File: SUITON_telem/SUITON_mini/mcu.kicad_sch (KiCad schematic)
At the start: 24 parts, among them J2 USB_C_Receptacle_USB2.0_14P, J4 Conn_01x06_Pin, U5 STM32F405RGT6, X1 ABM3B-8.000MHZ-10-1UT

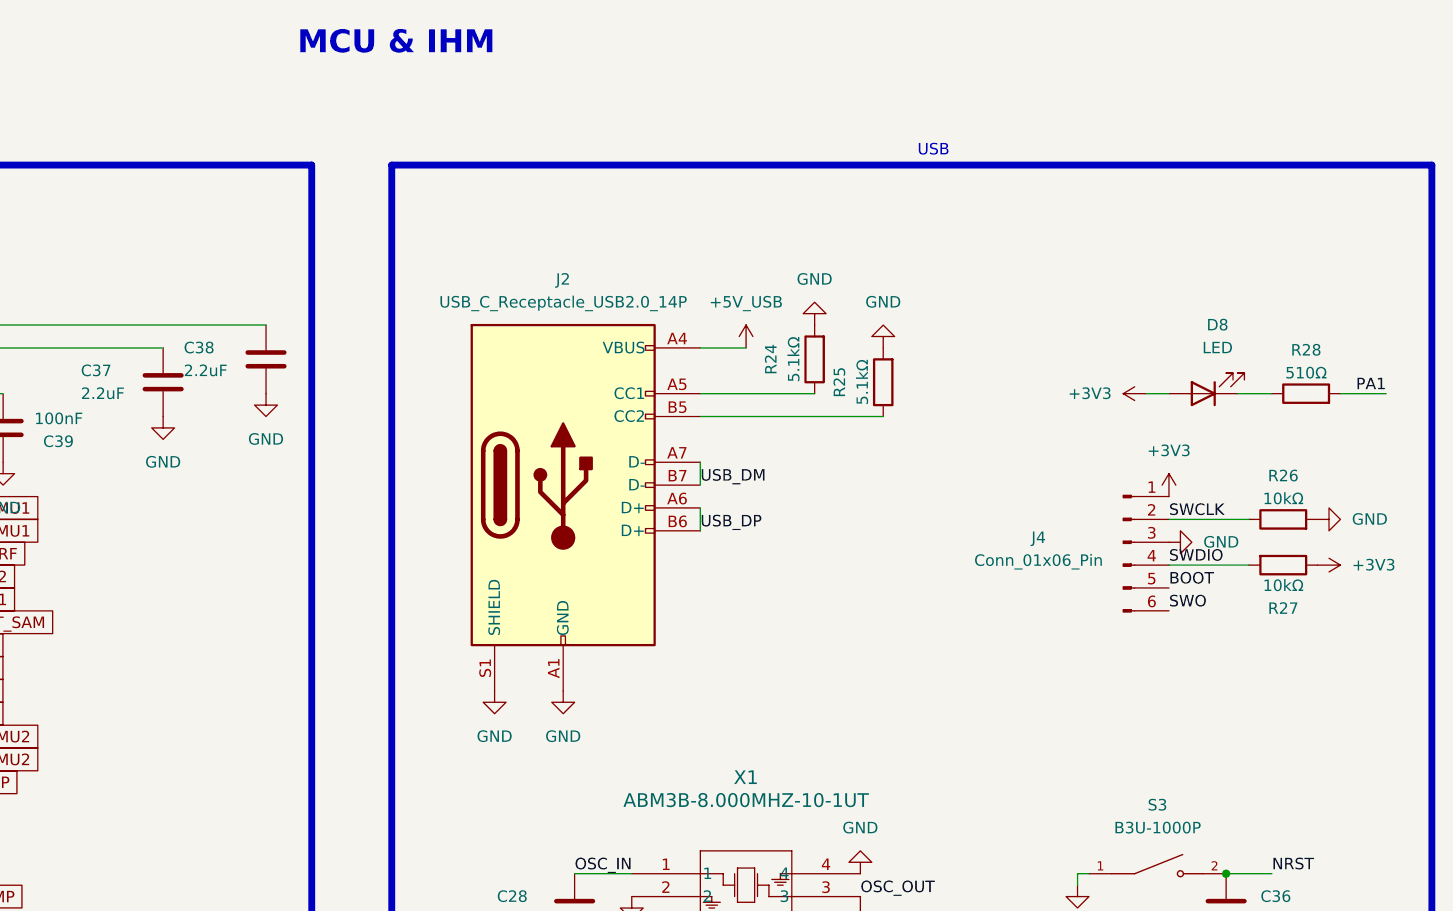
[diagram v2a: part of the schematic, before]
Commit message: Commencement du placement des composants
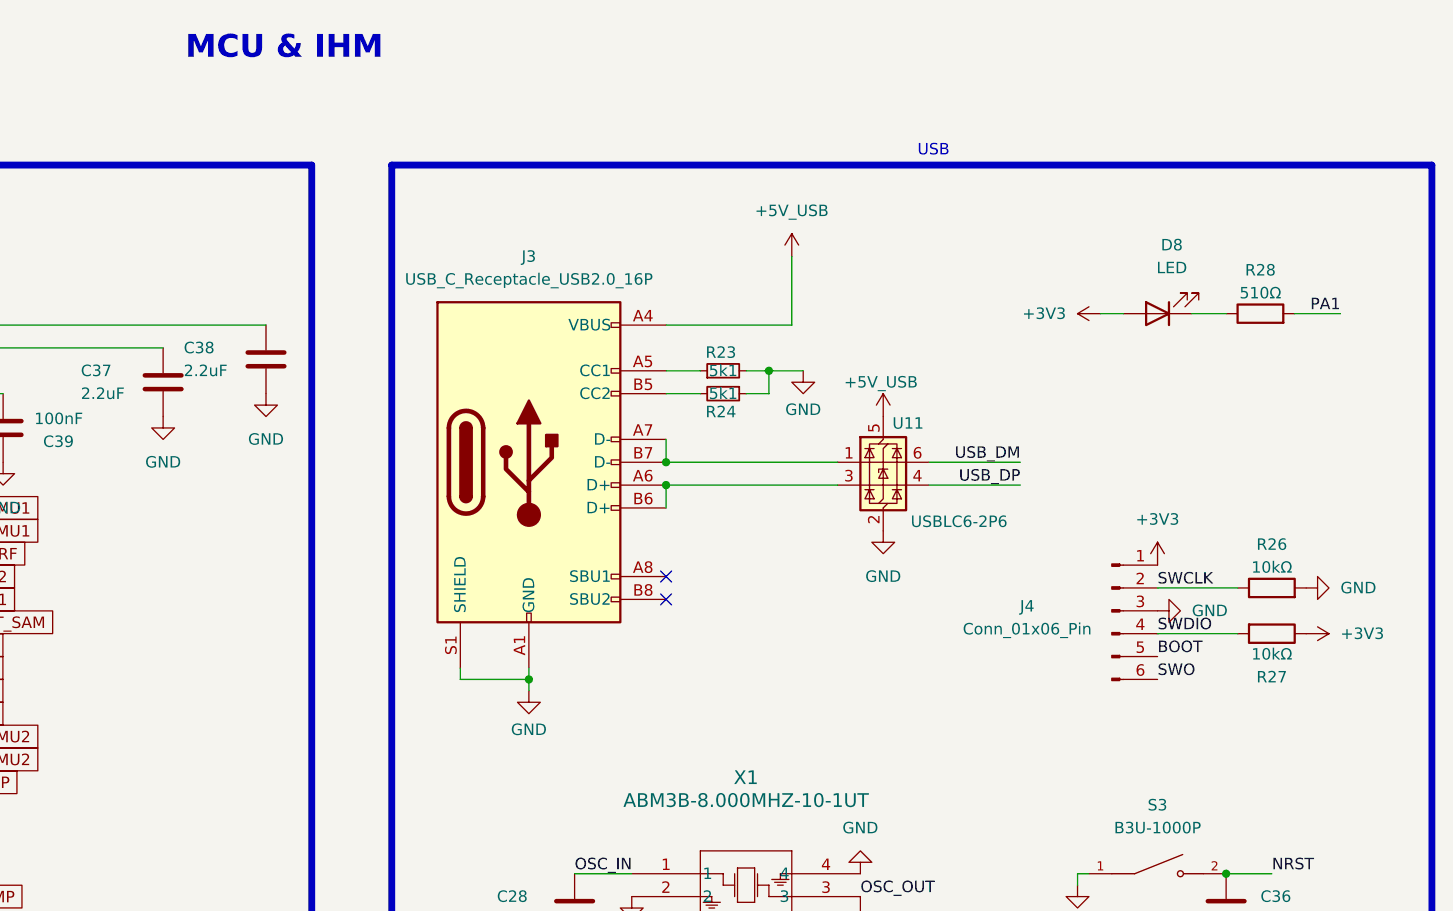
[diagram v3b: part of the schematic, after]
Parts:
- removed J2: USB_C_Receptacle_USB2.0_14P, symbol Connector:USB_C_Receptacle_USB2.0_14P
- removed R24, R25: 5.1kΩ, symbol Device:R
- added J3: USB_C_Receptacle_USB2.0_16P, Connector_USB:USB_C_Receptacle_GCT_USB4105-xx-A_16P_TopMnt_Horizontal, symbol Connector:USB_C_Receptacle_USB2.0_16P
- added R23, R24: 5k1, Resistor_SMD:R_0402_1005Metric, symbol Device:R_Small
- added U11: USBLC6-2P6, Package_TO_SOT_SMD:SOT-666, symbol Power_Protection:USBLC6-2P6
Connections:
- net +5V_USB: now also J3.A4 (VBUS), J3.A9 (VBUS), J3.B4 (VBUS), J3.B9 (VBUS), U11.5 (VBUS)
- net GND: now also J3.A1 (GND), J3.A12 (GND), J3.B1 (GND), J3.B12 (GND), J3.S1 (SHIELD), R23.2, R24.1, U11.2 (GND)
- net USB_DM: now also U11.6 (I/O1)
- net USB_DP: now also U11.4 (I/O2)
- new net: J3.A7 (D-), J3.B7 (D-), U11.1 (I/O1)
- new net: J3.A6 (D+), J3.B6 (D+), U11.3 (I/O2)
- new net: J3.A5 (CC1), R23.1
- new net: J3.B5 (CC2), R24.2
- no-connect marks 8 -> 10
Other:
- moved on the sheet: D8, J4, R26, R27, R28
